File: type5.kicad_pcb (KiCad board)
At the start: 2 copper layers, 87.5 x 66.2 mm, 3 parts, among them P1 CONN_01X09, P2 CONN_01X26, U1 TEENSYPP2

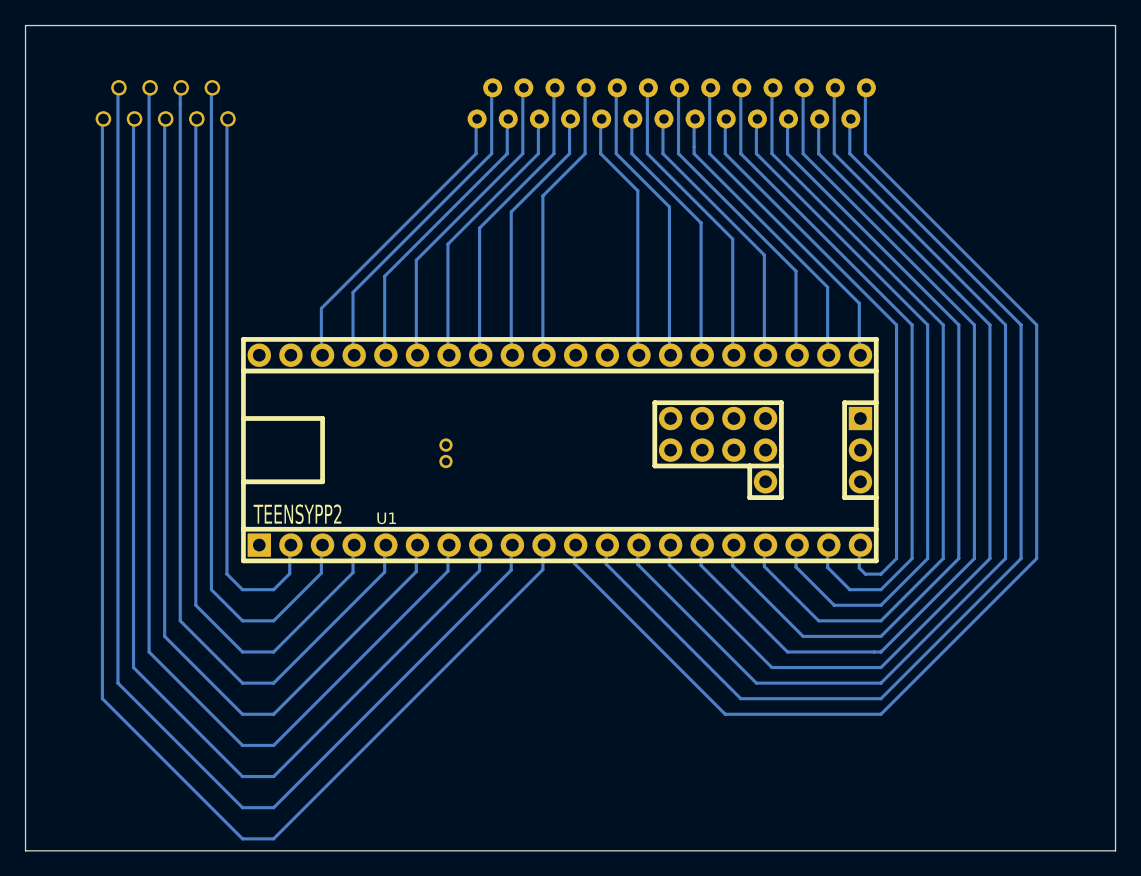
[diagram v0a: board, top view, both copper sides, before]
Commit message: mod
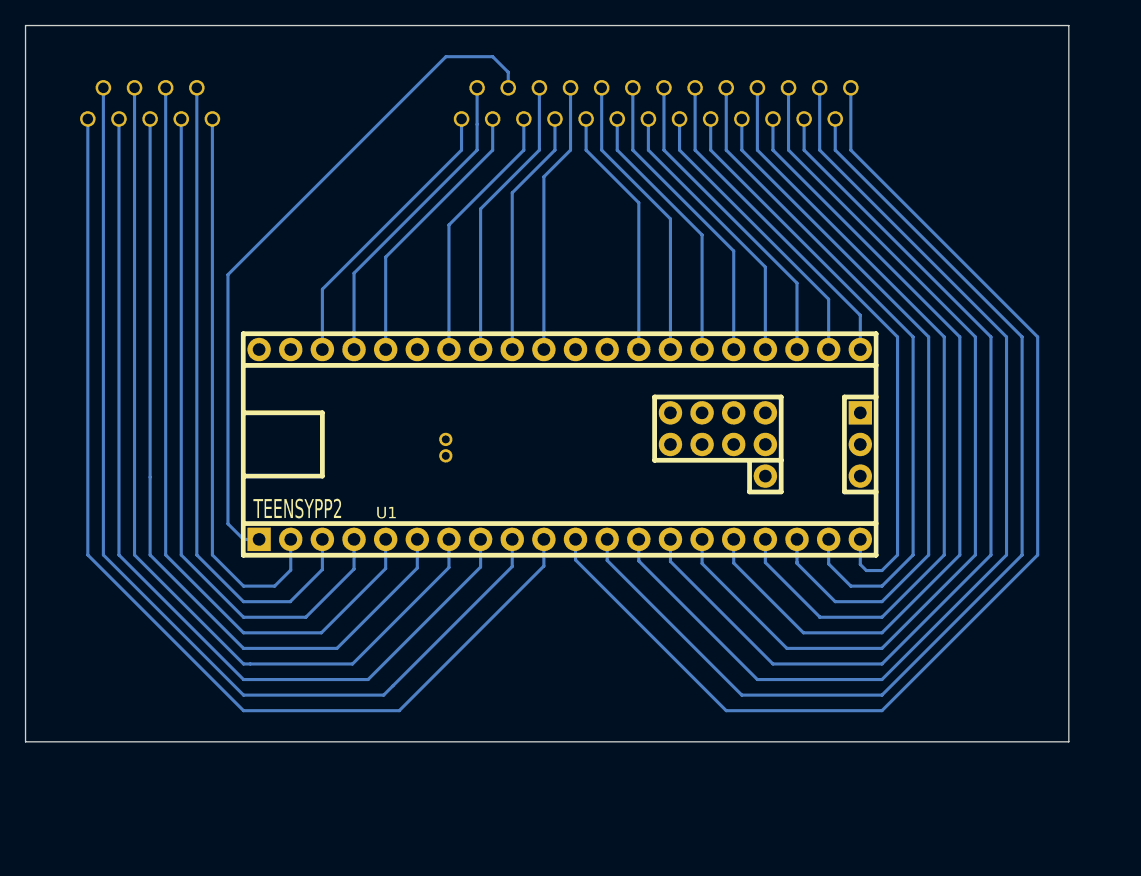
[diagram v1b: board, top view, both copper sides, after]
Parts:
- moved P1 1.25 mm to (110.0, 71.2)
- moved P2 1.25 mm to (150.0, 72.5)
- moved U1 0.46 mm to (142.9, 96.1)
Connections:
- U1 pad 1: Net-(U1-Pad1) -> Net-(P2-Pad4)
- U1 pad 47: Net-(P2-Pad4) -> Net-(U1-Pad47)
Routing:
- net Net-(P2-Pad4): track 24.8 -> 54.5 mm
- net Net-(P1-Pad1): track 97.1 -> 83.7 mm
- net Net-(P1-Pad2): track 93.1 -> 81.4 mm
- net Net-(P1-Pad3): track 84.0 -> 74.1 mm
- net Net-(P1-Pad4): track 79.9 -> 71.8 mm
- net Net-(P1-Pad5): track 70.8 -> 64.5 mm
- net Net-(P1-Pad6): track 66.8 -> 62.2 mm
- net Net-(P1-Pad7): track 57.7 -> 54.9 mm
- net Net-(P1-Pad8): track 53.6 -> 52.6 mm
- net Net-(P2-Pad22): track 72.7 -> 73.5 mm
- net Net-(P2-Pad21): track 65.4 -> 66.2 mm
- net Net-(P2-Pad20): track 63.1 -> 63.8 mm
- net Net-(P2-Pad17): track 46.2 -> 46.9 mm
- net Net-(P2-Pad25): track 84.6 -> 85.4 mm
- net Net-(P2-Pad24): track 82.3 -> 83.0 mm
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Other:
- board size 87.5 x 66.2 mm -> 83.8 x 57.5 mm
